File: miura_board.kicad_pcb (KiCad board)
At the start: 2 copper layers, 60 x 60 mm, 44 parts, among them J1 Screw_Terminal_01x02, J2 Screw_Terminal_01x02, J3 Screw_Terminal_01x02, J4 Conn_01x04_Male, J5 Screw_Terminal_01x02, J6 Screw_Terminal_01x02, J7 Screw_Terminal_01x02, J8 Screw_Terminal_01x02, SW1 SW_Push, SW2 SW_Push, U1 ESP32-WROOM, U3 DRV8833PW, U4 DRV8833PW, U5 AMS1117, U6 MPU-6050, U7 L7806, U8 DRV8833PW

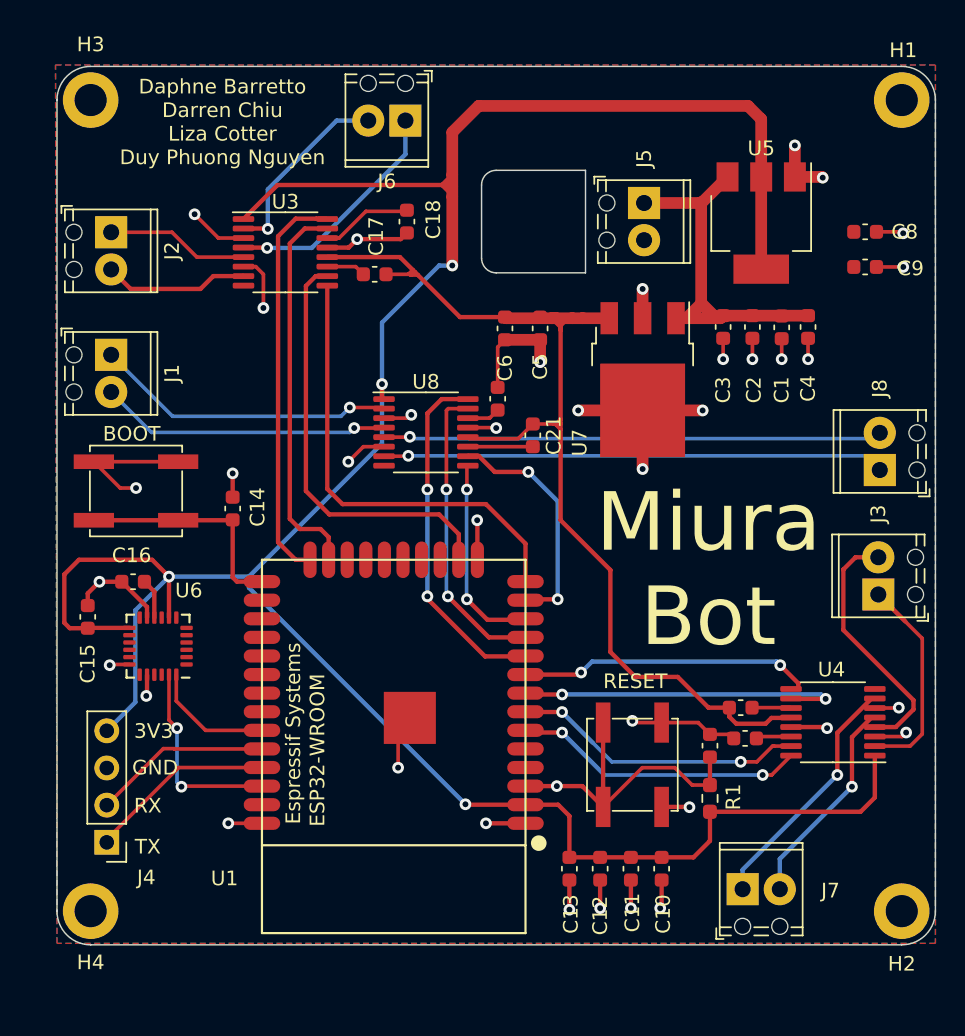
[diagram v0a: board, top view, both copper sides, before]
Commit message: new board design
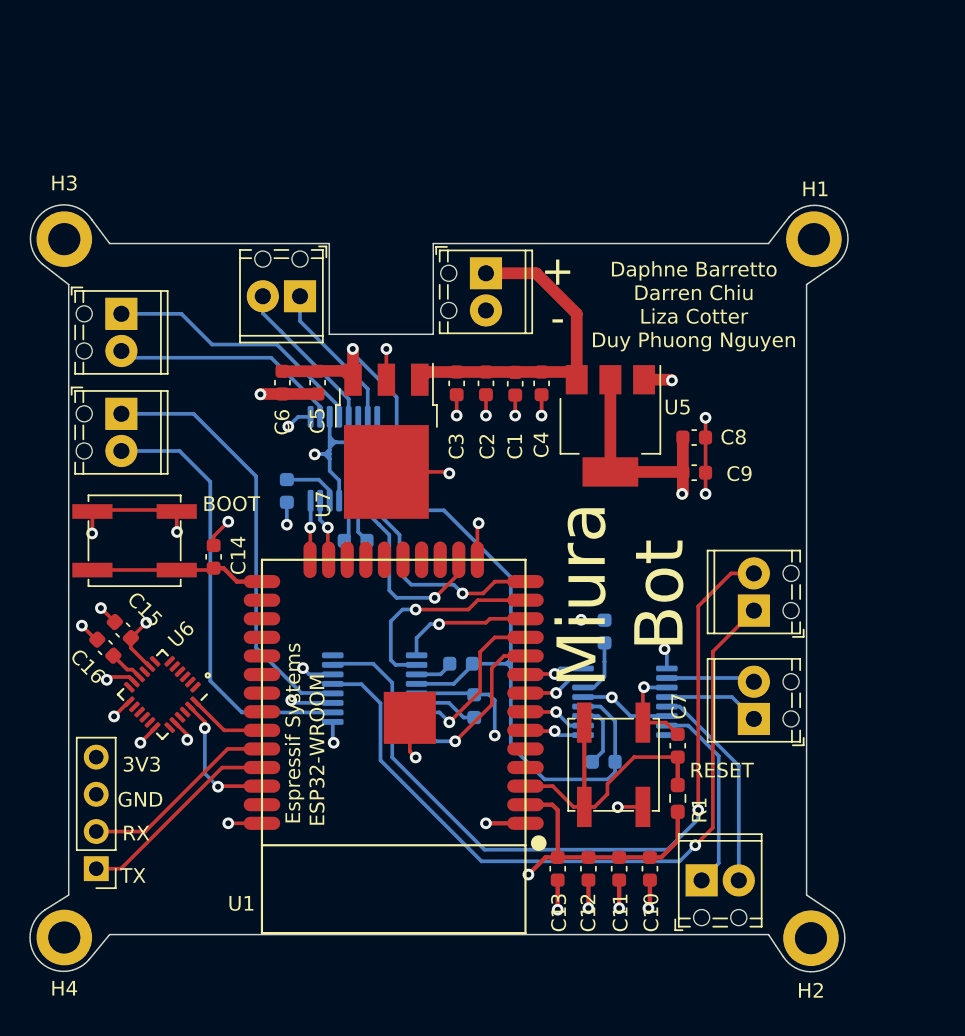
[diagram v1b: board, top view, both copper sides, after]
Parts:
- C17, C18, C19, C20, C21, C22, U3, U4, U8: moved to B.Cu
- moved C22 21.1 mm to (89.5, 68.7)
- moved C18 20.1 mm to (76.7, 54.0)
- moved C2 18.6 mm to (90.3, 46.6)
- moved C3 18.6 mm to (88.3, 46.6)
- moved C4 18.6 mm to (94.1, 46.6)
- moved C1 18.6 mm to (92.3, 46.7)
- moved C8 18.3 mm to (104.5, 50.4)
- moved C9 18.3 mm to (104.5, 52.8)
- moved C17 18.2 mm to (81.4, 57.4), turned to 0 degrees
- moved U7 18.0 mm to (83.5, 50.6)
- moved U8 17.8 mm to (82.7, 67.5)
- moved U5 17.3 mm to (98.8, 49.5)
- moved C21 16.4 mm to (88.6, 65.8), turned to 180 degrees
- moved C5 15.6 mm to (78.8, 46.6)
- moved C6 15.6 mm to (76.4, 46.6)
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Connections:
- net Net-(J7-Pad1) renamed /IO34
- net Net-(J7-Pad2) renamed /IO35
- J1 pad 1: Net-(J1-Pad1) -> /IO26
- J1 pad 2: Net-(J1-Pad2) -> /IO25
- J2 pad 1: Net-(J2-Pad1) -> /IO15
- J2 pad 2: Net-(J2-Pad2) -> /IO2
- J3 pad 1: Net-(U4-Pad2) -> /IO32
- J3 pad 2: Net-(U4-Pad4) -> /IO33
- J6 pad 1: Net-(J6-Pad1) -> /IO12
- J6 pad 2: Net-(J6-Pad2) -> /IO13
- J8 pad 1: Net-(J8-Pad1) -> /IO14
- J8 pad 2: Net-(J8-Pad2) -> /IO27
- U1 pad 6: MOTOR_A21_IN -> MOTOR_A22_IN
- U1 pad 7: MOTOR_A22_IN -> MOTOR_A21_IN
- U3 pad 2: Net-(J6-Pad2) -> /IO2
- U3 pad 4: Net-(J6-Pad1) -> /IO15
- U3 pad 5: Net-(J2-Pad1) -> /IO13
- U3 pad 7: Net-(J2-Pad2) -> /IO12
- U4 pad 10: MOTOR_B22_IN -> MOTOR_A21_IN
- U4 pad 15: MOTOR_A22_IN -> MOTOR_B22_IN
- U4 pad 16: MOTOR_A21_IN -> MOTOR_B21_IN
- U4 pad 2: Net-(U4-Pad2) -> /IO33
- U4 pad 4: Net-(U4-Pad4) -> /IO32
- U4 pad 9: MOTOR_B21_IN -> MOTOR_A22_IN
- U8 pad 2: Net-(J1-Pad1) -> /IO25
- U8 pad 4: Net-(J1-Pad2) -> /IO26
- U8 pad 5: Net-(J8-Pad2) -> /IO14
- U8 pad 7: Net-(J8-Pad1) -> /IO27
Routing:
- net +3V3: track 182.5 -> 43.9 mm, vias 4 -> 7
- net /IO27: track 0.00 -> 53.4 mm, vias 0 -> 1
- net /IO14: track 0.00 -> 50.2 mm, vias 0 -> 1
- net Net-(J8-Pad1): track 34.4 -> 0.00 mm, vias 1 -> 0
- net Net-(J8-Pad2): track 34.1 -> 0.00 mm, vias 1 -> 0
- net /IO25: track 0.00 -> 29.7 mm
- net /IO26: track 0.00 -> 29.1 mm
- net MOTOR_A11_IN: track 27.5 -> 4.03 mm, vias 0 -> 1
- net MOTOR_A12_IN: track 26.5 -> 4.28 mm, vias 0 -> 1
- net Net-(J1-Pad1): track 20.7 -> 0.00 mm, vias 1 -> 0
- net Net-(J1-Pad2): track 19.9 -> 0.00 mm, vias 1 -> 0
- net MOTOR_B22_IN: track 22.7 -> 4.36 mm, vias 2 -> 1
- net /IO15: track 0.00 -> 18.1 mm
- net Net-(U4-Pad2): track 17.0 -> 0.00 mm
- net Net-(U4-Pad4): track 16.9 -> 0.00 mm
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- added copper zone on In2.Cu, net +3V3
- added copper zone on In1.Cu, net GND
- removed copper zone on B.Cu, net GND
- removed copper zone on F.Cu, net GND
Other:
- board size 60 x 60 mm -> 55.9 x 52.4 mm
- copper layers 2 -> 4
- board text added: "+ -"
- board text added: "12 13"
- board text added: "15 2"
- board text added: "26 14"
- board text added: "26 25"
- board text added: "33 32"
- board text added: "34 35"
